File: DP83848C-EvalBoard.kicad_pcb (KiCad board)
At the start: 4 copper layers, 75 x 100 mm, 189 parts, among them J1 Conn_01x02, J10 Conn_02x04_Odd_Even, J11 Conn_02x04_Odd_Even, J12 Conn_02x04_Odd_Even, J13 Conn_02x04_Odd_Even, J14 Conn_02x04_Odd_Even, J2 RJ45_LED_Shielded, J3 USB_C_Receptacle_USB2.0, J4 Conn_02x05_Odd_Even, J5 Conn_01x04, J6 Conn_01x04, J7 Conn_01x04, J8 Conn_02x08_Odd_Even, J9 Conn_02x08_Odd_Even, Q1 AO3401A, Q2 AO3400A, Q3 AO3401A, SW1 SW_Push, T1 H1102NL, U1 AMS1117-3.3, U10 CM1224, U11 CM1224, U12 CM1224, U13 CM1224, U14 CM1224, U15 CM1224, U2 DP83848C, U3 STM32F407VGTx, U4 USBLC6-2SC6, U5 CM1224, U6 CM1224, U7 CM1224, U8 CM1224, U9 CM1224, X1 50MHz, Y1 25MHz

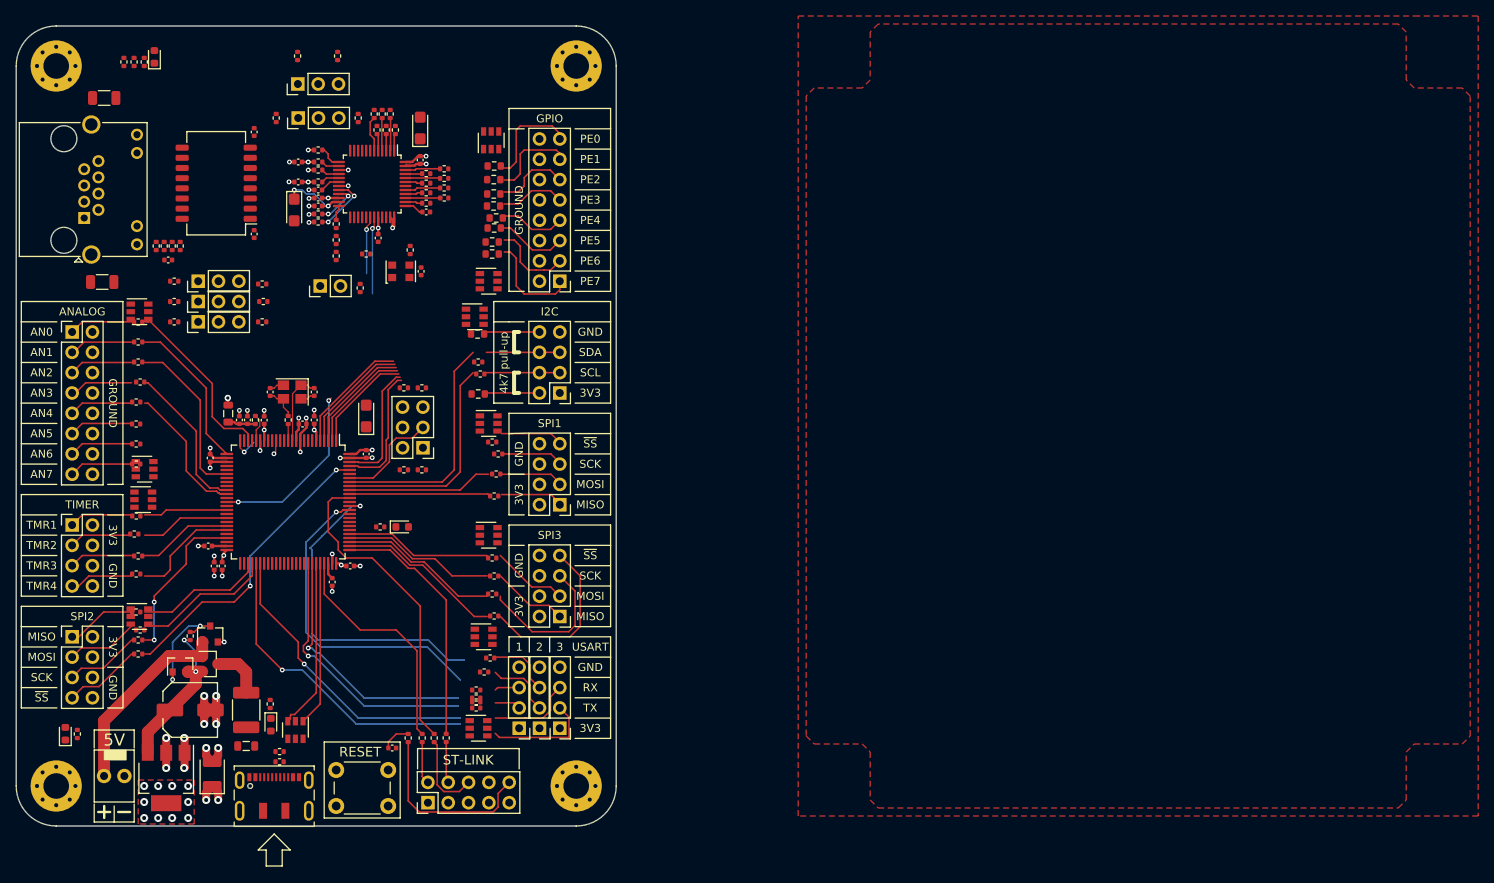
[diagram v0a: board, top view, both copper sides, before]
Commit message: Layout
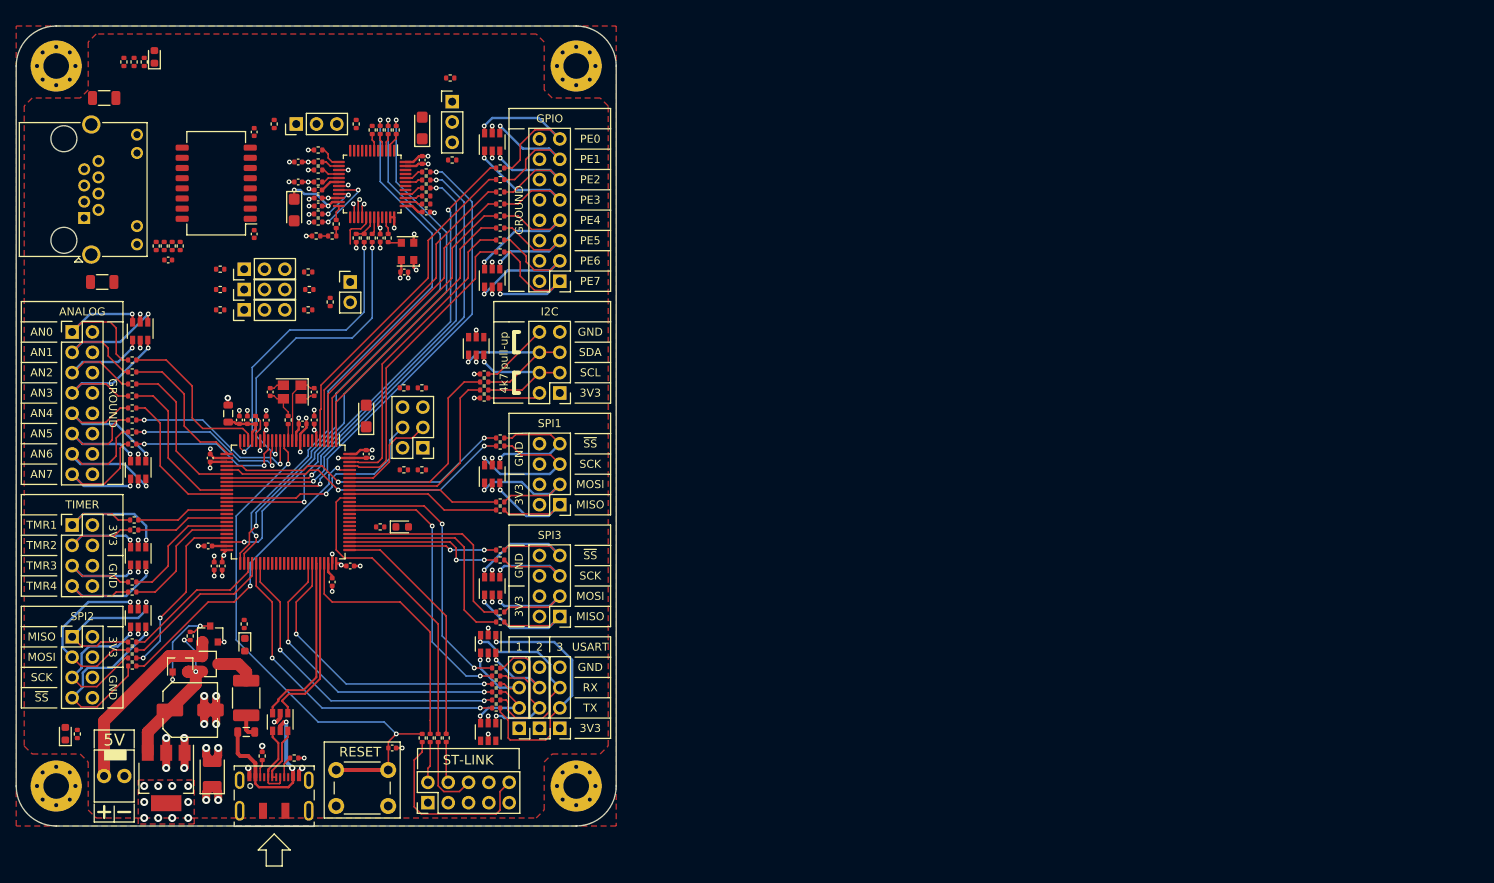
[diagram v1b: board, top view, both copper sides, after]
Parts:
- removed R16, R7, R9: 33, Resistor_SMD:R_0402_1005Metric
- R100, R101, R62, R63, R64, R65, R66, R67, R68, R69: footprint Resistor_SMD:R_0603_1608Metric -> Resistor_SMD:R_0402_1005Metric
- R19: value 1.5k -> 2.2k
- moved JP2 19.4 mm to (94.5, 66.5), turned to 0 degrees
- moved R31 19.3 mm to (94.5, 73.8), turned to 180 degrees
- moved R30 19.3 mm to (94.2, 63.5), turned to 180 degrees
- moved R14 13.2 mm to (83.5, 83.5), turned to 270 degrees
- moved D2 10.5 mm to (68.6, 134.3)
- moved R3 10.5 mm to (68.5, 131.8)
- moved R13 10.5 mm to (84.5, 83.5), turned to 270 degrees
- moved R93 8.28 mm to (100.5, 122.5)
- moved U14 7.07 mm to (55.2, 123.2), turned to 270 degrees
- moved R91 6.82 mm to (100.5, 130.2)
- moved U12 6.37 mm to (99.5, 127.0), turned to 90 degrees
- moved U6 6.34 mm to (99.5, 113.0), turned to 90 degrees
- moved JP4 5.94 mm to (68.5, 92.5)
- moved JP5 5.94 mm to (68.5, 89.9)
- moved JP6 5.94 mm to (68.5, 87.4)
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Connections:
- J11 pad 7: /IO/SPI1_NSS -> /IO/SPI1_NSS_R
- J3 pad A8: Net-(J3-PadA8) -> (no net)
- J3 pad B8: Net-(J3-PadB8) -> (no net)
- J4 pad 7: Net-(J4-Pad7) -> (no net)
- J4 pad 8: Net-(J4-Pad8) -> (no net)
- R13 pad 2: /PHY/RXD_2 -> /ETH_MDC
- R14 pad 2: /PHY/RXD_3 -> /ETH_MDIO
- R15 pad 2: /PHY/RX_CLK -> (no net)
- R19 pad 1: /ETH_MDIO -> Net-(R14-Pad1)
- R85 pad 1: /IO/SPI1_NSS -> /IO/SPI1_NSS_R
- U10 pad 1: /IO/USART3_TX_R -> /IO/USART2_TX_R
- U10 pad 3: /IO/USART3_RX_R -> /IO/USART1_TX_R
- U10 pad 4: Net-(U10-Pad4) -> (no net)
- U10 pad 6: Net-(U10-Pad6) -> (no net)
- U11 pad 1: /IO/ADC0_R -> /IO/ADC1_R
- U11 pad 3: /IO/ADC1_R -> /IO/ADC0_R
- U13 pad 1: /IO/I2C1_SCL_R -> /IO/I2C1_SDA_R
- U13 pad 3: /IO/I2C1_SDA_R -> /IO/I2C1_SCL_R
- U13 pad 4: Net-(U13-Pad4) -> (no net)
- U13 pad 6: Net-(U13-Pad6) -> (no net)
- U15 pad 4: /IO/ADC6_R -> /IO/ADC7_R
- U15 pad 6: /IO/ADC7_R -> /IO/ADC6_R
- U2 pad 1: Net-(R9-Pad1) -> (no net)
- U2 pad 25: Net-(U2-Pad25) -> (no net)
- U2 pad 30: /ETH_MDIO -> Net-(R14-Pad1)
- U2 pad 31: /ETH_MDC -> Net-(R13-Pad1)
- U2 pad 33: Net-(U2-Pad33) -> (no net)
- U2 pad 41: Net-(R16-Pad1) -> (no net)
- U2 pad 42: Net-(U2-Pad42) -> (no net)
- U2 pad 45: Net-(R13-Pad1) -> (no net)
- U2 pad 46: Net-(R14-Pad1) -> (no net)
- U2 pad 5: Net-(R7-Pad1) -> (no net)
- U2 pad 7: Net-(U2-Pad7) -> (no net)
- U3 pad 24: /MCU/ETH_REF_CLK -> (no net)
- U3 pad 39: Net-(U3-Pad39) -> (no net)
- U3 pad 41: Net-(U3-Pad41) -> (no net)
- U3 pad 43: Net-(U3-Pad43) -> (no net)
- U3 pad 46: Net-(U3-Pad46) -> (no net)
- U3 pad 57: Net-(U3-Pad57) -> (no net)
- U3 pad 58: Net-(U3-Pad58) -> (no net)
- U3 pad 59: Net-(U3-Pad59) -> (no net)
- U3 pad 60: Net-(U3-Pad60) -> (no net)
- U3 pad 61: Net-(U3-Pad61) -> (no net)
- U3 pad 62: Net-(U3-Pad62) -> (no net)
- U3 pad 63: Net-(U3-Pad63) -> (no net)
- U3 pad 64: Net-(U3-Pad64) -> (no net)
- U3 pad 65: Net-(U3-Pad65) -> (no net)
- U3 pad 66: Net-(U3-Pad66) -> (no net)
- U3 pad 67: Net-(U3-Pad67) -> (no net)
- U3 pad 7: Net-(U3-Pad7) -> (no net)
- U3 pad 8: Net-(U3-Pad8) -> (no net)
- U3 pad 82: Net-(U3-Pad82) -> (no net)
- U3 pad 83: Net-(U3-Pad83) -> (no net)
- U3 pad 84: Net-(U3-Pad84) -> (no net)
- U3 pad 85: Net-(U3-Pad85) -> (no net)
- U3 pad 88: Net-(U3-Pad88) -> (no net)
- U3 pad 9: Net-(U3-Pad9) -> (no net)
- U3 pad 95: Net-(U3-Pad95) -> (no net)
- U5 pad 1: /IO/GPIO0_R -> /IO/GPIO1_R
- U5 pad 3: /IO/GPIO1_R -> /IO/GPIO0_R
- U6 pad 1: /IO/SPI1_MISO_R -> /IO/SPI1_MOSI_R
- U6 pad 3: /IO/SPI1_MOSI_R -> /IO/SPI1_MISO_R
- U6 pad 4: /IO/SPI1_SCK_R -> /IO/SPI1_NSS_R
- U6 pad 6: /IO/SPI1_NSS -> /IO/SPI1_SCK_R
- U7 pad 1: /IO/USART1_TX_R -> /IO/USART3_TX_R
- U7 pad 3: /IO/USART1_RX_R -> /IO/USART3_RX_R
- U7 pad 4: /IO/USART2_TX_R -> /IO/USART1_RX_R
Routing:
- net /ETH_TX_EN: track 0.00 -> 69.8 mm, vias 0 -> 2
- net /ETH_TX_D0: track 0.00 -> 69.2 mm, vias 0 -> 2
- net /ETH_TX_D1: track 0.00 -> 69.1 mm, vias 0 -> 2
- net /MCU/NRST: track 3.66 -> 67.4 mm, vias 0 -> 2
- net /ETH_RXD1: track 0.00 -> 61.7 mm, vias 0 -> 2
- net /ETH_RXD0: track 0.00 -> 59.0 mm, vias 0 -> 2
- net /ETH_CRS_DV: track 0.00 -> 56.3 mm, vias 0 -> 2
- net /IO/GPIO7: track 22.4 -> 62.0 mm
- net /IO/SPI1_SCK: track 0.00 -> 37.4 mm, vias 0 -> 2
- net /IO/SPI1_NSS: track 7.96 -> 37.2 mm, vias 0 -> 2
- net /ETH_MDC: track 11.4 -> 39.4 mm
- net /MCU/BOOT1: track 0.00 -> 27.7 mm, vias 0 -> 1
- net /ETH_MDIO: track 10.6 -> 38.2 mm
- net /IO/GPIO6: track 15.1 -> 42.3 mm
- net /IO/GPIO5: track 14.5 -> 40.6 mm
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- added copper zone on F.Cu, net (none)
- removed copper zone on F.Cu, net GNDPWR
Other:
- rule pad_to_mask_clearance: 0 -> 0.05
